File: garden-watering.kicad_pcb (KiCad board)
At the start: 2 copper layers, 65 x 90 mm, 65 parts, among them J1 Barrel_Jack, J10 Conn_01x04, J11 Conn_01x05, J2 Conn_01x03, J3 Screw_Terminal_01x02, J4 Screw_Terminal_01x02, J5 Screw_Terminal_01x02, J6 Screw_Terminal_01x02, J7 Conn_01x04, J8 Conn_01x04, J9 Conn_01x04, K1 SANYOU_SRD_Form_C, K2 SANYOU_SRD_Form_C, K3 SANYOU_SRD_Form_C, K4 SANYOU_SRD_Form_C, Q1 2N2222, Q2 2N2222, Q3 2N2222, Q4 2N2222, SW1 SW_SPDT, SW2 SW_SPDT, SW3 SW_SPDT, SW4 SW_SPDT, U1 LM2576HVT-3.3, U2 ESP32-WROOM-32, U3 DHT11

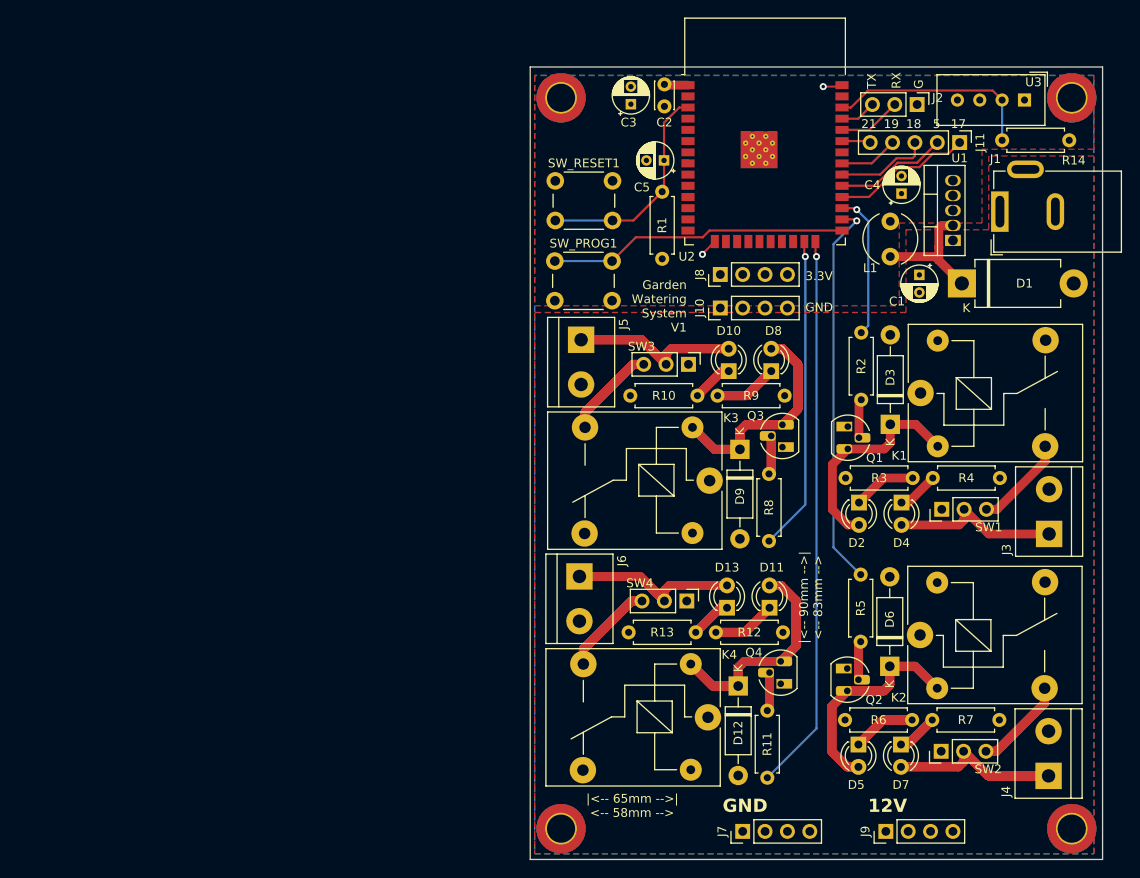
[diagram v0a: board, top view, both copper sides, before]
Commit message: misc
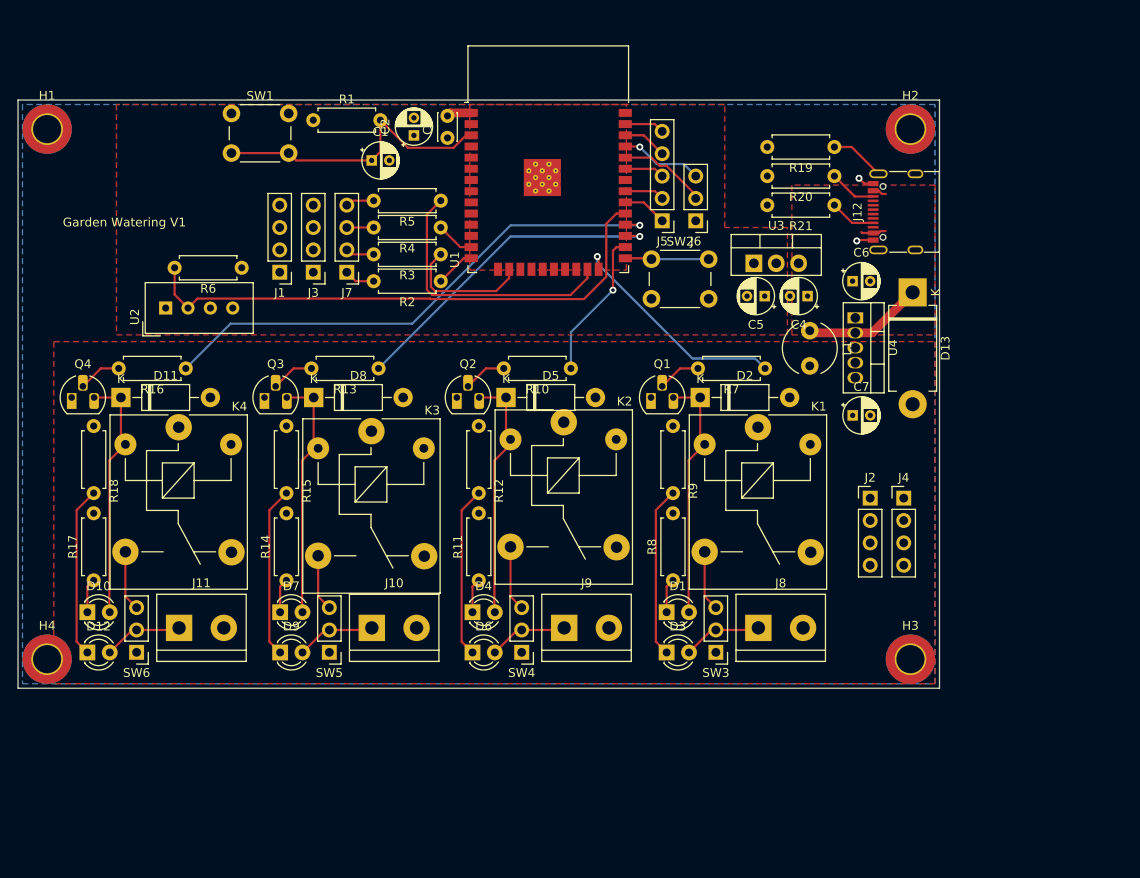
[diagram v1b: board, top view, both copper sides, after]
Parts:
- removed SW_PROG1, SW_RESET1: SW_Push, Button_Switch_THT:SW_PUSH_6mm
- added C6: 100uF, Capacitor_THT:CP_Radial_D4.0mm_P2.00mm, F.Cu at (193.6, 68.3)
- added C7: 220uF, Capacitor_THT:CP_Radial_D4.0mm_P2.00mm, F.Cu at (193.6, 83.6)
- added J12: USB_C_Receptacle, Connector_USB:USB_C_Receptacle_G-Switch_GT-USB-7010ASV, F.Cu at (199.6, 60.5)
- added R15: 220R, Resistor_THT:R_Axial_DIN0207_L6.3mm_D2.5mm_P7.62mm_Horizontal, F.Cu at (129.3, 92.4)
- added R16: 1K, Resistor_THT:R_Axial_DIN0207_L6.3mm_D2.5mm_P7.62mm_Horizontal, F.Cu at (117.9, 78.2)
- added R17: 220R, Resistor_THT:R_Axial_DIN0207_L6.3mm_D2.5mm_P7.62mm_Horizontal, F.Cu at (107.4, 102.3)
- added R18: 220R, Resistor_THT:R_Axial_DIN0207_L6.3mm_D2.5mm_P7.62mm_Horizontal, F.Cu at (107.4, 92.4)
- added R19: 1M, Resistor_THT:R_Axial_DIN0207_L6.3mm_D2.5mm_P7.62mm_Horizontal, F.Cu at (191.5, 53.1)
- added R20: 5.11K, Resistor_THT:R_Axial_DIN0207_L6.3mm_D2.5mm_P7.62mm_Horizontal, F.Cu at (191.5, 56.4)
- added R21: 5.11K, Resistor_THT:R_Axial_DIN0207_L6.3mm_D2.5mm_P7.62mm_Horizontal, F.Cu at (191.5, 59.7)
- added SW5: SW_SPDT, Connector_PinHeader_2.54mm:PinHeader_1x03_P2.54mm_Vertical, F.Cu at (134.2, 110.5)
- added SW6: SW_SPDT, Connector_PinHeader_2.54mm:PinHeader_1x03_P2.54mm_Vertical, F.Cu at (112.3, 110.5)
- added U4: LM2576T-12, Package_TO_SOT_THT:TO-220-5_Vertical, F.Cu at (193.9, 72.5)
- C1: value 100uF -> 1uF
- C2: value 100nF -> 10uF; footprint Capacitor_THT:C_Disc_D3.0mm_W2.0mm_P2.50mm -> Capacitor_THT:CP_Radial_D4.0mm_P2.00mm
- C3: value 10uF -> 100nF; footprint Capacitor_THT:CP_Radial_D4.0mm_P2.00mm -> Capacitor_THT:C_Disc_D3.0mm_W2.0mm_P2.50mm
- C4: value 1000uF -> 10uF
- C5: value 1uF -> 100uF
- D1: value MBR360 -> LED; footprint Diode_THT:D_DO-201AD_P12.70mm_Horizontal -> LED_THT:LED_D3.0mm
- D11, D2, D5, D8: value LED -> 1N4007; footprint LED_THT:LED_D3.0mm -> Diode_THT:D_DO-41_SOD81_P10.16mm_Horizontal
- D12, D3, D6, D9: value 1N4007 -> LED; footprint Diode_THT:D_DO-41_SOD81_P10.16mm_Horizontal -> LED_THT:LED_D3.0mm
- D13: value LED -> D_Schottky; footprint LED_THT:LED_D3.0mm -> Diode_THT:D_DO-201AD_P12.70mm_Horizontal
- J1: value Barrel_Jack -> GND; footprint Connector_BarrelJack:BarrelJack_GCT_DCJ200-10-A_Horizontal -> Connector_PinHeader_2.54mm:PinHeader_1x04_P2.54mm_Vertical
- J10, J8, J9: value Conn_01x04 -> Screw_Terminal_01x02; footprint Connector_PinHeader_2.54mm:PinHeader_1x04_P2.54mm_Vertical -> TerminalBlock:TerminalBlock_bornier-2_P5.08mm
- J11: value Conn_01x05 -> Screw_Terminal_01x02; footprint Connector_PinHeader_2.54mm:PinHeader_1x05_P2.54mm_Vertical -> TerminalBlock:TerminalBlock_bornier-2_P5.08mm
- J2: value Conn_01x03 -> GND; footprint Connector_PinHeader_2.54mm:PinHeader_1x03_P2.54mm_Vertical -> Connector_PinHeader_2.54mm:PinHeader_1x04_P2.54mm_Vertical
- J3: value Screw_Terminal_01x02 -> +3.3V; footprint TerminalBlock:TerminalBlock_bornier-2_P5.08mm -> Connector_PinHeader_2.54mm:PinHeader_1x04_P2.54mm_Vertical
- J4: value Screw_Terminal_01x02 -> +12V; footprint TerminalBlock:TerminalBlock_bornier-2_P5.08mm -> Connector_PinHeader_2.54mm:PinHeader_1x04_P2.54mm_Vertical
- J5: value Screw_Terminal_01x02 -> GPIO; footprint TerminalBlock:TerminalBlock_bornier-2_P5.08mm -> Connector_PinHeader_2.54mm:PinHeader_1x05_P2.54mm_Vertical
- J6: value Screw_Terminal_01x02 -> UART; footprint TerminalBlock:TerminalBlock_bornier-2_P5.08mm -> Connector_PinHeader_2.54mm:PinHeader_1x03_P2.54mm_Vertical
- J7: value Conn_01x04 -> JTAG
- R10, R13, R7: value 220R -> 1K
- R11, R8: value 1K -> 220R
- R14: value 10K -> 220R
- R2, R5: value 1K -> 100R
- R3, R4: value 220R -> 100R
- R6: value 220R -> 10K
- SW1: value SW_SPDT -> RESET; footprint Connector_PinHeader_2.54mm:PinHeader_1x03_P2.54mm_Vertical -> Button_Switch_THT:SW_PUSH_6mm
- SW2: value SW_SPDT -> PROG; footprint Connector_PinHeader_2.54mm:PinHeader_1x03_P2.54mm_Vertical -> Button_Switch_THT:SW_PUSH_6mm
- U1: value LM2576HVT-3.3 -> ESP32-WROOM-32; footprint Package_TO_SOT_THT:TO-220-5_Vertical -> RF_Module:ESP32-WROOM-32
- U2: value ESP32-WROOM-32 -> DHT11; footprint RF_Module:ESP32-WROOM-32 -> Sensor:Aosong_DHT11_5.5x12.0_P2.54mm
- U3: value DHT11 -> LM1117T-3.3; footprint Sensor:Aosong_DHT11_5.5x12.0_P2.54mm -> Package_TO_SOT_THT:TO-220-3_Vertical
- moved H4 132.7 mm to (102.1, 111.3)
- moved J11 104.4 mm to (117.1, 107.7), turned to 0 degrees
- moved R14 102.0 mm to (129.3, 102.3), turned to 90 degrees
- moved SW1 92.4 mm to (123.0, 49.3), turned to 0 degrees
- moved R6 91.8 mm to (124.2, 66.8)
- moved H2 88.8 mm to (200.2, 51.1)
- moved J3 88.7 mm to (132.3, 67.3), turned to 180 degrees
- moved Q4 86.8 mm to (104.9, 81.5), turned to 0 degrees
- moved J1 82.1 mm to (128.5, 67.3), turned to 180 degrees
- moved D10 77.8 mm to (106.7, 105.9), turned to 0 degrees
- moved J7 77.8 mm to (136.1, 67.3), turned to 180 degrees
- moved D11 77.4 mm to (110.5, 81.5), turned to 0 degrees
- moved D12 74.0 mm to (106.7, 110.5), turned to 0 degrees
- moved D7 72.1 mm to (128.6, 105.9), turned to 0 degrees
- moved U2 70.2 mm to (115.6, 71.4), turned to 90 degrees
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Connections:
- C1 pad 1: +12V -> Net-(U1-EN)
- C4 pad 1: +3.3V -> VBUS
- C5 pad 1: Net-(U2-EN) -> +3.3V
- D1 pad 2: GND -> Net-(D1-A)
- D11 pad 1: Net-(D11-K) -> Net-(D10-A)
- D11 pad 2: Net-(D11-A) -> GND
- D12 pad 1: Net-(D11-A) -> Net-(D12-K)
- D12 pad 2: GND -> Net-(D12-A)
- D13 pad 2: Net-(D13-A) -> GND
- D2 pad 1: Net-(D2-K) -> Net-(D1-A)
- D2 pad 2: Net-(D2-A) -> GND
- D3 pad 1: Net-(D2-A) -> Net-(D3-K)
- D3 pad 2: GND -> Net-(D3-A)
- D5 pad 1: Net-(D5-K) -> Net-(D4-A)
- D5 pad 2: Net-(D5-A) -> GND
- D6 pad 1: Net-(D5-A) -> Net-(D6-K)
- D6 pad 2: GND -> Net-(D6-A)
- D8 pad 1: Net-(D8-K) -> Net-(D7-A)
- D8 pad 2: Net-(D8-A) -> GND
- D9 pad 1: Net-(D8-A) -> Net-(D9-K)
- D9 pad 2: GND -> Net-(D9-A)
- J1 pad 1: +12V -> GND
- J1 pad 3: (no net) -> GND
- J10 pad 1: GND -> Net-(D9-A)
- J11 pad 1: IO17 -> Net-(D12-A)
- J11 pad 2: IO5 -> GND
- J2 pad 2: RX -> GND
- J2 pad 3: TX -> GND
- J3 pad 1: Net-(D4-A) -> +3.3V
- J3 pad 2: GND -> +3.3V
- J4 pad 1: Net-(D7-A) -> +12V
- J4 pad 2: GND -> +12V
- J5 pad 1: Net-(D10-A) -> IO18
- J5 pad 2: GND -> IO19
- J6 pad 1: Net-(D13-A) -> GND
- J6 pad 2: GND -> RX
- J7 pad 1: GND -> Net-(J7-Pin_1)
- J7 pad 2: GND -> Net-(J7-Pin_2)
- J7 pad 3: GND -> Net-(J7-Pin_3)
- J7 pad 4: GND -> Net-(J7-Pin_4)
- J8 pad 1: +3.3V -> Net-(D3-A)
- J8 pad 2: +3.3V -> GND
- J9 pad 1: +12V -> Net-(D6-A)
- J9 pad 2: +12V -> GND
- K1 pad 2: Net-(D2-A) -> Net-(D1-A)
- K1 pad 3: Net-(SW1-C) -> Net-(SW3-C)
- K2 pad 2: Net-(D5-A) -> Net-(D4-A)
- K2 pad 3: Net-(SW2-C) -> Net-(SW4-C)
- K3 pad 2: Net-(D8-A) -> Net-(D7-A)
- K3 pad 3: Net-(SW3-C) -> Net-(SW5-C)
- K4 pad 2: Net-(D11-A) -> Net-(D10-A)
- K4 pad 3: Net-(SW4-C) -> Net-(SW6-C)
- L1 pad 1: Net-(D1-K) -> Net-(D13-K)
- L1 pad 2: +3.3V -> +12V
- Q1 pad 3: Net-(D2-A) -> Net-(D1-A)
- Q2 pad 3: Net-(D5-A) -> Net-(D4-A)
- Q3 pad 3: Net-(D8-A) -> Net-(D7-A)
- Q4 pad 3: Net-(D11-A) -> Net-(D10-A)
- R1 pad 2: Net-(U2-EN) -> Net-(U1-EN)
- R10 pad 1: Net-(D10-K) -> RELAY_2
- R10 pad 2: GND -> Net-(Q2-B)
- R11 pad 1: RELAY_4 -> Net-(D4-K)
- R11 pad 2: Net-(Q4-B) -> GND
- R12 pad 1: Net-(D11-K) -> Net-(D6-K)
- R13 pad 1: Net-(D13-K) -> RELAY_3
- R13 pad 2: GND -> Net-(Q3-B)
- R14 pad 1: +3.3V -> Net-(D7-K)
- R14 pad 2: DHT -> GND
- R2 pad 1: RELAY_1 -> MTDI
- R2 pad 2: Net-(Q1-B) -> Net-(J7-Pin_1)
- R3 pad 1: Net-(D2-K) -> MTCK
- R3 pad 2: GND -> Net-(J7-Pin_2)
- R4 pad 1: Net-(D4-K) -> MTMS
- R4 pad 2: GND -> Net-(J7-Pin_3)
- R5 pad 1: RELAY_2 -> MTDO
- R5 pad 2: Net-(Q2-B) -> Net-(J7-Pin_4)
- R6 pad 1: Net-(D5-K) -> +3.3V
- R6 pad 2: GND -> DHT
- R7 pad 1: Net-(D7-K) -> RELAY_1
- R7 pad 2: GND -> Net-(Q1-B)
- R8 pad 1: RELAY_3 -> Net-(D1-K)
- R8 pad 2: Net-(Q3-B) -> GND
- R9 pad 1: Net-(D8-K) -> Net-(D3-K)
- SW1 pad 1: +12V -> GND
- SW1 pad 2: Net-(D4-A) -> Net-(U1-EN)
- SW2 pad 1: +12V -> Net-(U1-IO0)
- SW2 pad 2: Net-(D7-A) -> GND
- SW3 pad 2: Net-(D10-A) -> Net-(D3-A)
- SW4 pad 2: Net-(D13-A) -> Net-(D6-A)
- U1 pad 1: +12V -> GND
- U1 pad 2: Net-(D1-K) -> +3.3V
- U1 pad 3: GND -> Net-(U1-EN)
- U1 pad 4: +3.3V -> unconnected-(U1-SENSOR_VP-Pad4)
- U1 pad 5: GND -> unconnected-(U1-SENSOR_VN-Pad5)
- U2 pad 1: GND -> +3.3V
- U2 pad 2: +3.3V -> DHT
- U2 pad 3: Net-(U2-EN) -> unconnected-(U2-NC-Pad3)
- U2 pad 4: unconnected-(U2-SENSOR_VP-Pad4) -> GND
- U3 pad 1: +3.3V -> GND
- U3 pad 2: DHT -> +3.3V
- U3 pad 3: unconnected-(U3-NC-Pad3) -> VBUS
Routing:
- net Net-(D8-A): track 100.0 -> 0.00 mm
- net Net-(D11-A): track 100.0 -> 0.00 mm
- net Net-(D5-A): track 97.5 -> 0.00 mm
- net Net-(D13-A): track 60.3 -> 0.00 mm
- net Net-(SW2-C): track 42.5 -> 0.00 mm
- net DHT: track 24.0 -> 62.9 mm
- net Net-(SW4-C): track 42.5 -> 6.86 mm
- net Net-(SW3-C): track 42.5 -> 6.86 mm
- net Net-(U2-IO0): track 34.1 -> 0.00 mm
- net Net-(U1-EN): track 0.00 -> 33.5 mm
- net Net-(D10-A): track 60.3 -> 28.4 mm
- net Net-(D7-A): track 60.3 -> 28.4 mm
- net MTDO: track 0.00 -> 31.0 mm
- net Net-(D11-K): track 29.0 -> 0.00 mm
- net Net-(D8-K): track 29.0 -> 0.00 mm
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- added copper zone on F.Cu, net GND
- added copper zone on F.Cu, net VBUS
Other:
- board size 65 x 90 mm -> 104.6 x 66.8 mm
- board text added: "Garden Watering V1"
- board text removed: "12V"
- board text removed: "17"
- board text removed: "18"
- board text removed: "19"
- board text removed: "21"
- board text removed: "3.3V"
- board text removed: "5"
- board text removed: "G"
- board text removed: "GND"
- board text removed: "Garden Watering System V1"
- board text removed: "RX"
- board text removed: "TX"
- board text removed: "|<-- 65mm -->| <-- 58mm -->"
- board text removed: "|<-- 90mm -->| <-- 83mm -->"
